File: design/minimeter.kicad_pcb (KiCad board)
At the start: 2 copper layers, 12 parts, among them J1 Conn_01x02_Pin, J2 I2C, SW1 SW_Push_Dual, SW2 SW_Push_Dual

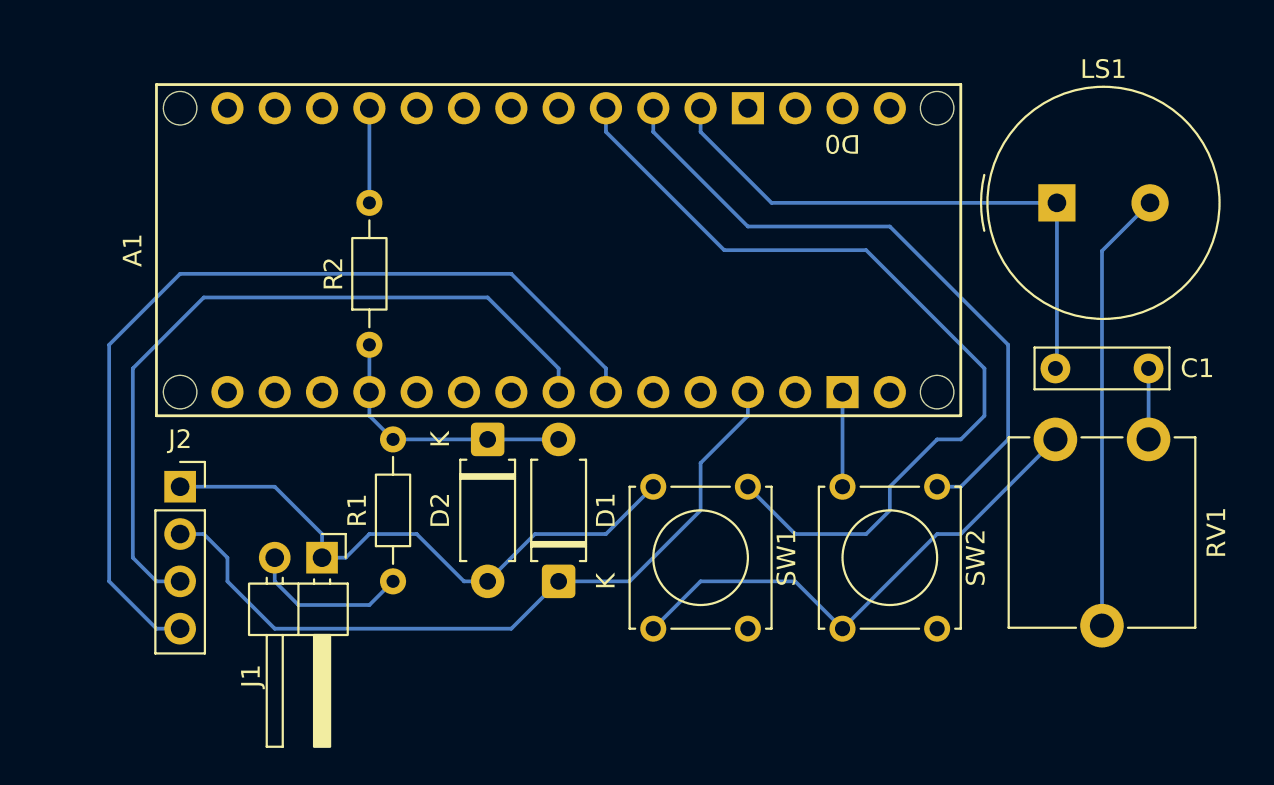
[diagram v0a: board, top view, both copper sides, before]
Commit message: Iterate on PCB
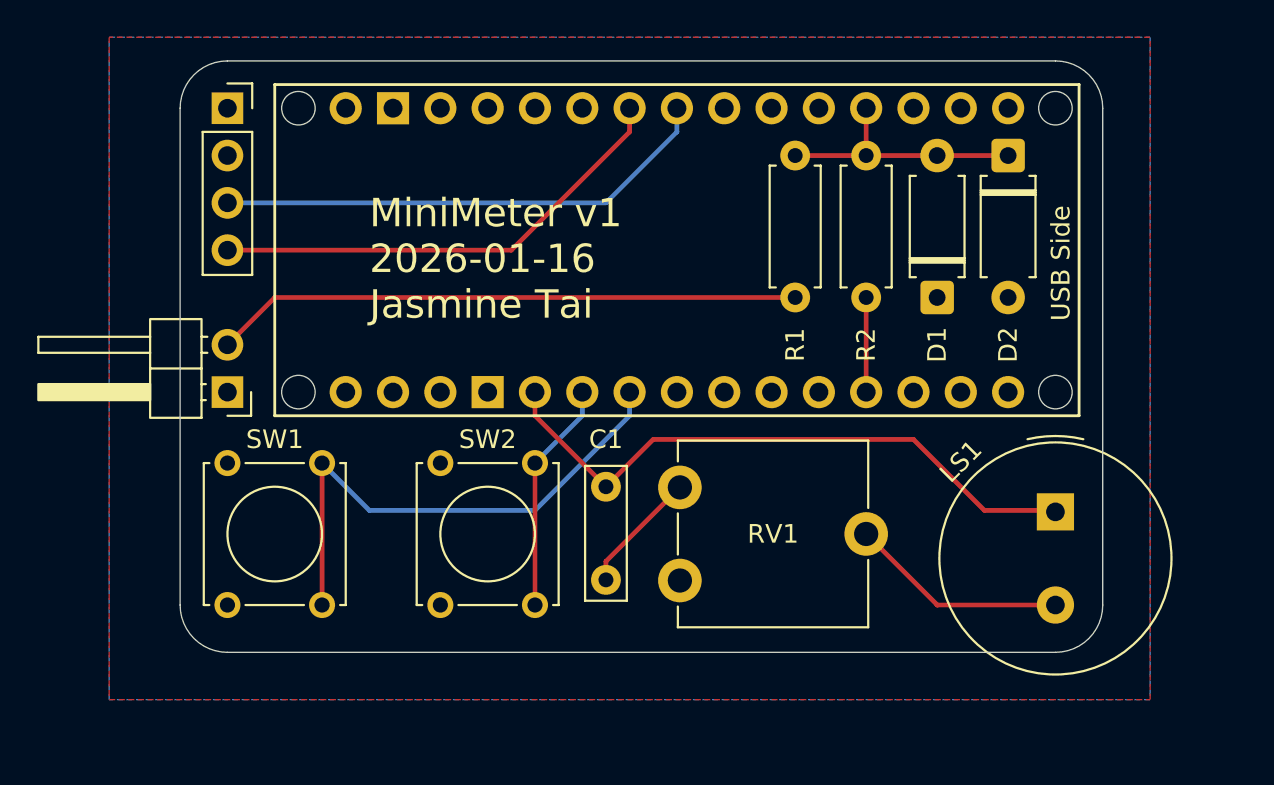
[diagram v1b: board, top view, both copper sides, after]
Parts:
- R1, R2: footprint Resistor_THT:R_Axial_DIN0204_L3.6mm_D1.6mm_P7.62mm_Horizontal -> Resistor_THT:R_Axial_DIN0207_L6.3mm_D2.5mm_P7.62mm_Horizontal
- moved A1 49.5 mm to (90.2, 57.1), turned to 90 degrees
- moved D2 31.8 mm to (86.4, 52.1)
- moved R2 28.5 mm to (78.7, 52.1), turned to -90 degrees
- moved R1 26.4 mm to (74.9, 59.7)
- moved D1 25.4 mm to (82.5, 59.7)
- moved C1 25.0 mm to (64.8, 69.8), turned to -90 degrees
- moved SW1 22.9 mm to (49.5, 68.6)
- moved SW2 21.6 mm to (61.0, 68.6)
- moved RV1 21.5 mm to (68.7, 74.9), turned to 0 degrees
- moved J2 20.5 mm to (44.5, 49.5)
- moved LS1 16.6 mm to (88.9, 71.2), turned to -90 degrees
- moved J1 10.2 mm to (44.5, 64.8), turned to 180 degrees
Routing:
- net GND: track 64.4 -> 0.00 mm
- net VCC: track 40.8 -> 0.00 mm
- net /SCL: track 49.2 -> 25.5 mm
- net /IN: track 8.67 -> 31.5 mm
- net /BTN_2: track 35.0 -> 12.5 mm
- net /BTN_1: track 46.5 -> 28.6 mm
- net /SDA: track 40.5 -> 27.0 mm
- net Net-(LS1-Pad2): track 23.8 -> 11.7 mm
- net Net-(C1-Pad2): track 3.81 -> 6.61 mm
- net /SPKR: track 30.9 -> 33.4 mm
- net /IN_PROT: track 14.5 -> 14.0 mm
- added copper zone on F.Cu, net GND
- added copper zone on B.Cu, net VCC
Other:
- board outline added: 49.5 x 31.7 mm
- board text added: "MiniMeter v1 2026-01-16 Jasmine Tai"
- board text added: "USB Side"

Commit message: Iterate on PCB again
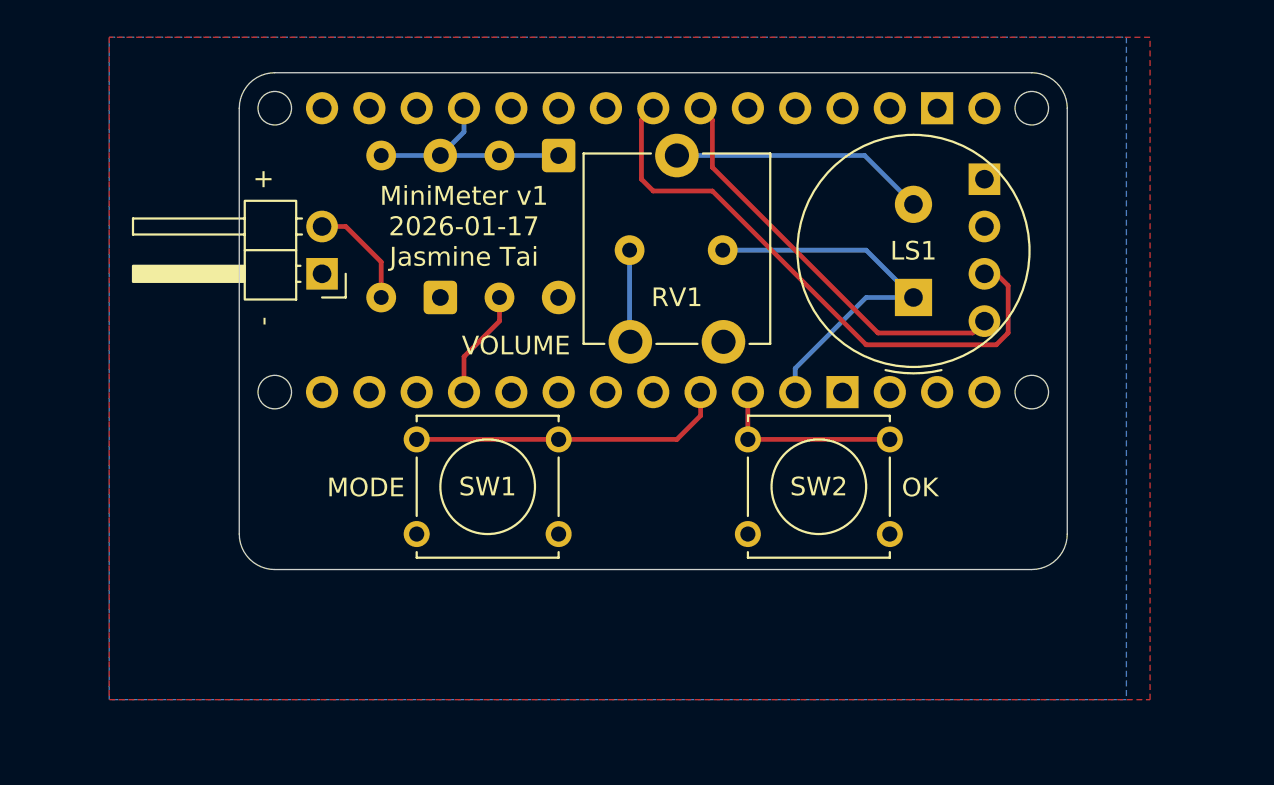
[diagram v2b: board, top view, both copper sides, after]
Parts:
- A1, C1, D1, D2, R1, R2: moved to B.Cu
- J2: footprint Connector_PinSocket_2.54mm:PinSocket_1x04_P2.54mm_Vertical -> Connector_PinSocket_2.54mm:PinSocket_1x04_P2.54mm_Horizontal; moved to B.Cu
- moved A1 44.5 mm to (45.7, 57.1)
- moved J2 40.8 mm to (85.1, 53.3), turned to 180 degrees
- moved D1 26.7 mm to (55.9, 59.7)
- moved D2 24.1 mm to (62.2, 52.1)
- moved R1 22.2 mm to (52.7, 59.7)
- moved R2 19.7 mm to (59.1, 52.1)
- moved C1 14.2 mm to (71.0, 57.1), turned to 180 degrees
- moved LS1 13.8 mm to (81.3, 59.7), turned to 90 degrees
- moved RV1 13.0 mm to (71.1, 62.1), turned to 90 degrees
- moved SW2 11.5 mm to (72.4, 67.3), turned to 0 degrees
- moved J1 8.13 mm to (49.5, 58.4)
- moved SW1 5.24 mm to (54.6, 67.3), turned to 0 degrees
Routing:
- net /IN: track 31.5 -> 5.87 mm
- net /SPKR: track 33.4 -> 20.5 mm
- net /BTN_1: track 28.6 -> 17.0 mm
- net /SDA: track 27.0 -> 31.8 mm
- net /SCL: track 25.5 -> 22.0 mm
- net /BTN_2: track 12.5 -> 10.2 mm
- net Net-(LS1-Pad2): track 11.7 -> 13.8 mm
- net Net-(C1-Pad2): track 6.61 -> 4.98 mm
- net /IN_PROT: track 14.0 -> 12.6 mm
- net /PULL: track 5.08 -> 5.87 mm
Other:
- board size 49.5 x 31.7 mm -> 44.4 x 26.7 mm
- board text added: "+"
- board text added: "-"
- board text added: "Copyright © 2026 Jasmine Tai. All rights reserved."
- board text added: "MODE"
- board text added: "MiniMeter v1 2026-01-17 Jasmine Tai"
- board text added: "OK"
- board text added: "USB SIDE"
- board text added: "VOLUME"
- board text added: "← I²C LCD"
- board text removed: "MiniMeter v1 2026-01-16 Jasmine Tai"
- board text removed: "USB Side"
